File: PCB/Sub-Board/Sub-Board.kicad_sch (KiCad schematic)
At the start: 0 parts

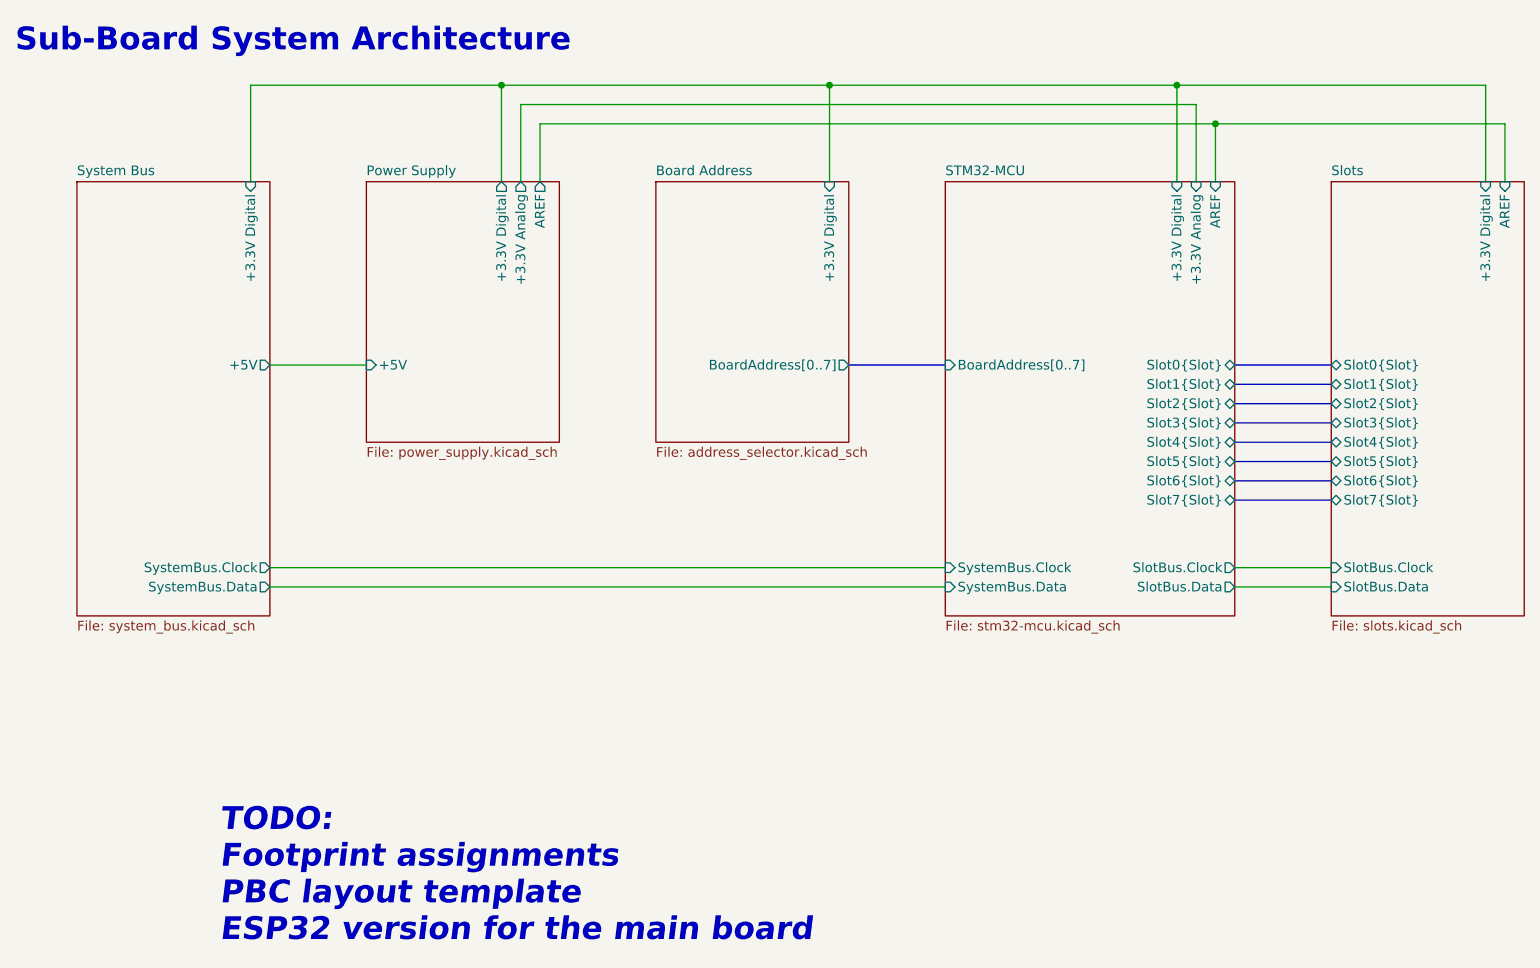
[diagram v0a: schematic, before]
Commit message: Sub-Board PCB: I2C Busses
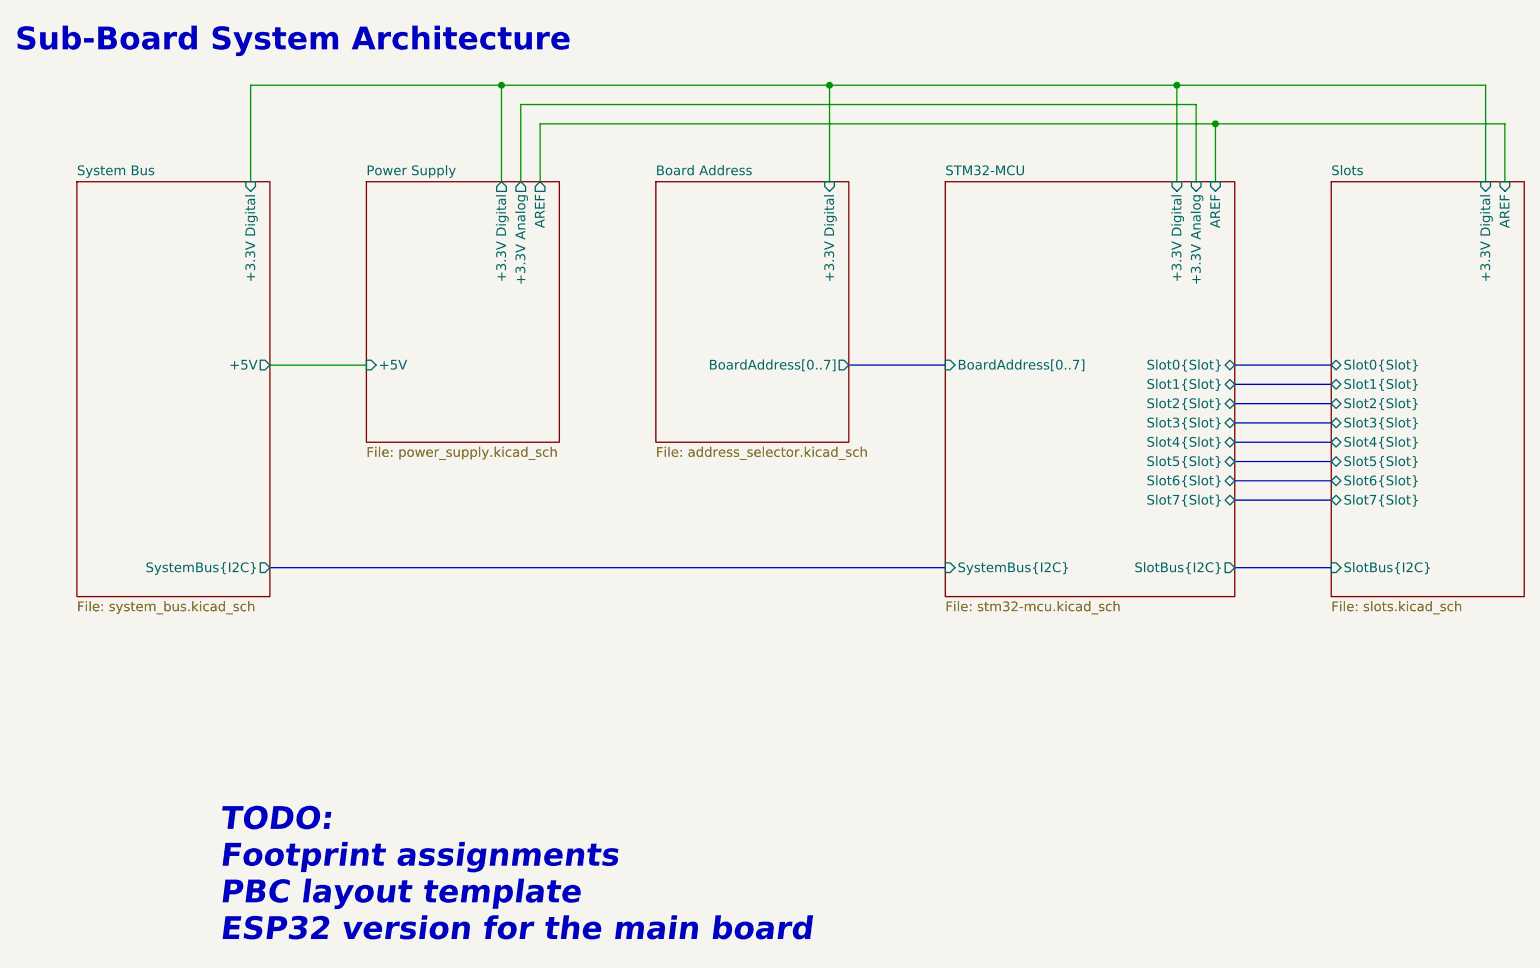
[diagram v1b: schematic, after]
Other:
- sheet STM32-MCU ports: added SlotBus{I2C}, SystemBus{I2C}; removed SlotBus.Clock, SlotBus.Data, SystemBus.Clock, SystemBus.Data
- sheet Slots ports: added SlotBus{I2C}; removed SlotBus.Clock, SlotBus.Data
- sheet System Bus ports: added SystemBus{I2C}; removed SystemBus.Clock, SystemBus.Data
